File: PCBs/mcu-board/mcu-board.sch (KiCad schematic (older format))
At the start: 22 parts, among them J5 MDAC-INPUT-SELECTOR, U1 m0-express, U2 SN74AHCT125DR, U3 SN74AHCT125DR

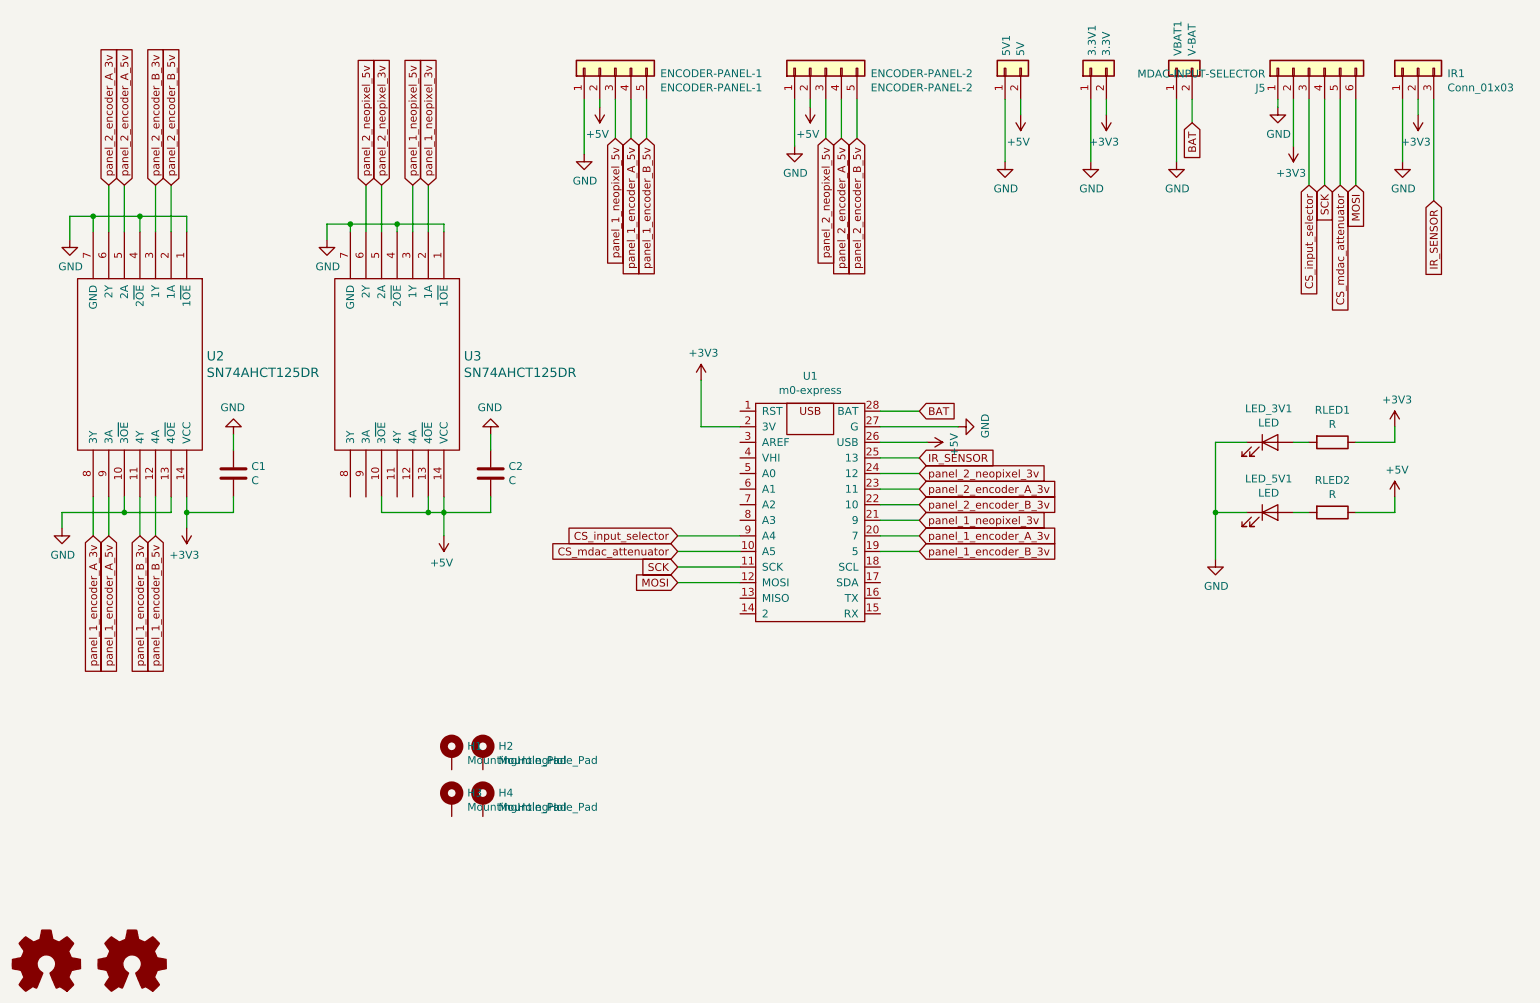
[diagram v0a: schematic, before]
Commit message: misc updates
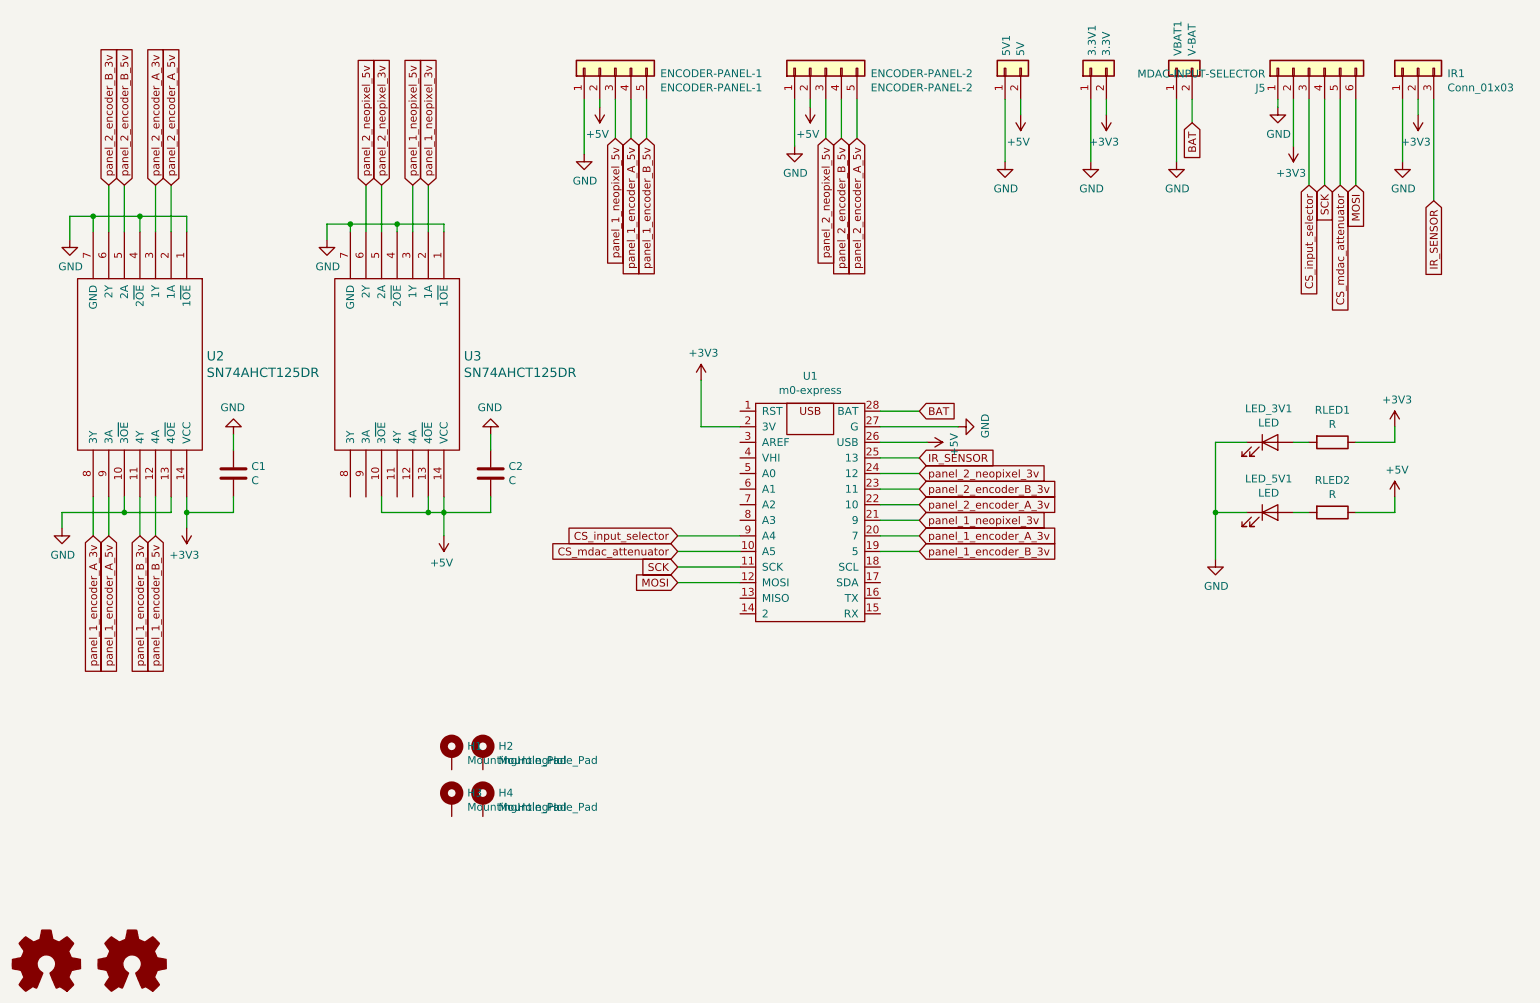
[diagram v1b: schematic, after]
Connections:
- net panel_2_encoder_A_3v: now also U1.22 (10), U2.3 (1Y); no longer U1.23 (11), U2.6 (2Y)
- net panel_2_encoder_A_5v: now also ENCODER-PANEL-2.5 (Pin_5), U2.2 (1A); no longer ENCODER-PANEL-2.4 (Pin_4), U2.5 (2A)
- net panel_2_encoder_B_3v: now also U1.23 (11), U2.6 (2Y); no longer U1.22 (10), U2.3 (1Y)
- net panel_2_encoder_B_5v: now also ENCODER-PANEL-2.4 (Pin_4), U2.5 (2A); no longer ENCODER-PANEL-2.5 (Pin_5), U2.2 (1A)
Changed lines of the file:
@@
 $EndComp
 Text GLabel 1500 2350 1    50   Input ~ 0
+panel_2_encoder_B_5v
+Text GLabel 1800 2350 1    50   Input ~ 0
 panel_2_encoder_A_5v
-Text GLabel 1800 2350 1    50   Input ~ 0
-panel_2_encoder_B_5v
 Wire Wire Line
 	1500 2650 1500 2350
@@
 	1800 2650 1800 2350
 Text GLabel 1400 2350 1    50   Input ~ 0
+panel_2_encoder_B_3v
+Text GLabel 1700 2350 1    50   Input ~ 0
 panel_2_encoder_A_3v
-Text GLabel 1700 2350 1    50   Input ~ 0
+Text GLabel 6600 4400 2    50   Input ~ 0
+panel_2_encoder_A_3v
+Text GLabel 6600 4300 2    50   Input ~ 0
 panel_2_encoder_B_3v
-Text GLabel 6600 4400 2    50   Input ~ 0
-panel_2_encoder_B_3v
-Text GLabel 6600 4300 2    50   Input ~ 0
-panel_2_encoder_A_3v
 Text GLabel 1300 4600 3    50   Input ~ 0
 panel_1_encoder_A_3v
@@
 panel_1_neopixel_5v
 Text GLabel 6200 2050 3    50   Input ~ 0
+panel_2_encoder_A_5v
+Text GLabel 6100 2050 3    50   Input ~ 0
 panel_2_encoder_B_5v
-Text GLabel 6100 2050 3    50   Input ~ 0
-panel_2_encoder_A_5v
 Text GLabel 4850 2050 3    50   Input ~ 0
 panel_1_encoder_B_5v
